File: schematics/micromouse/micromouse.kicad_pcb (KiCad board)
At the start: 2 copper layers, 207.5 x 125.6 mm, 13 parts, among them J1 TOF_FRONT, J2 TOF_LEFT, J3 TOF_RIGHT, J4 Conn_01x06, J5 BatteryConnector, U1 STM32F103CBTx, U2 PMW3360DM-T2QU, U3 BMI160, Y1 Crystal

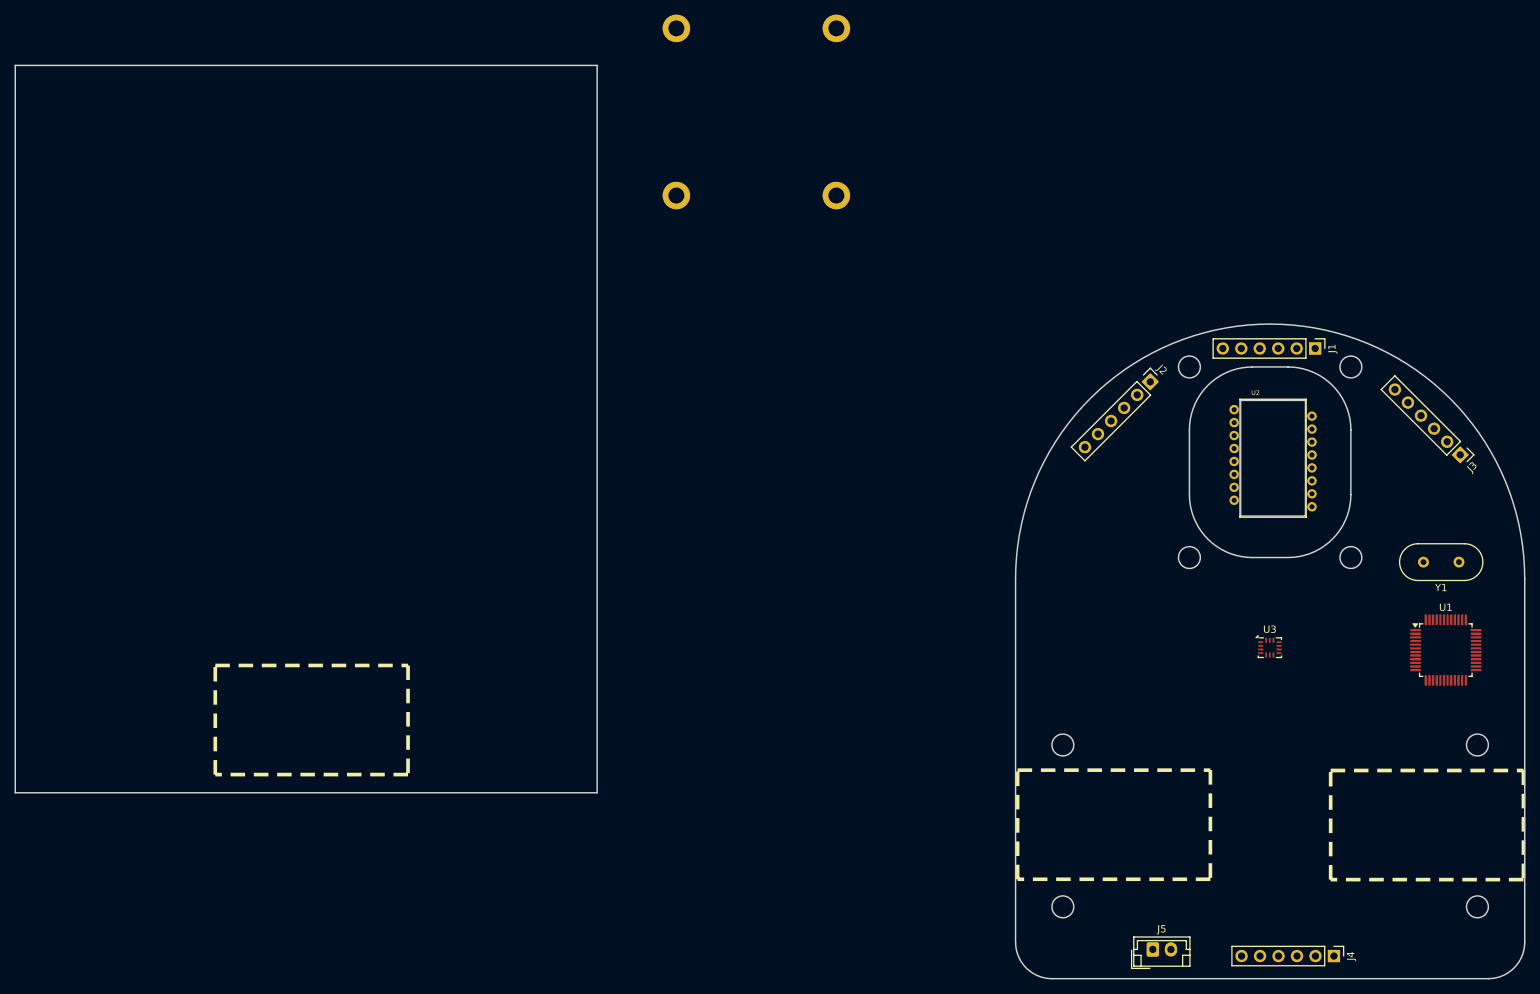
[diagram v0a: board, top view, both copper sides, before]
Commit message: Reorganize again... add things
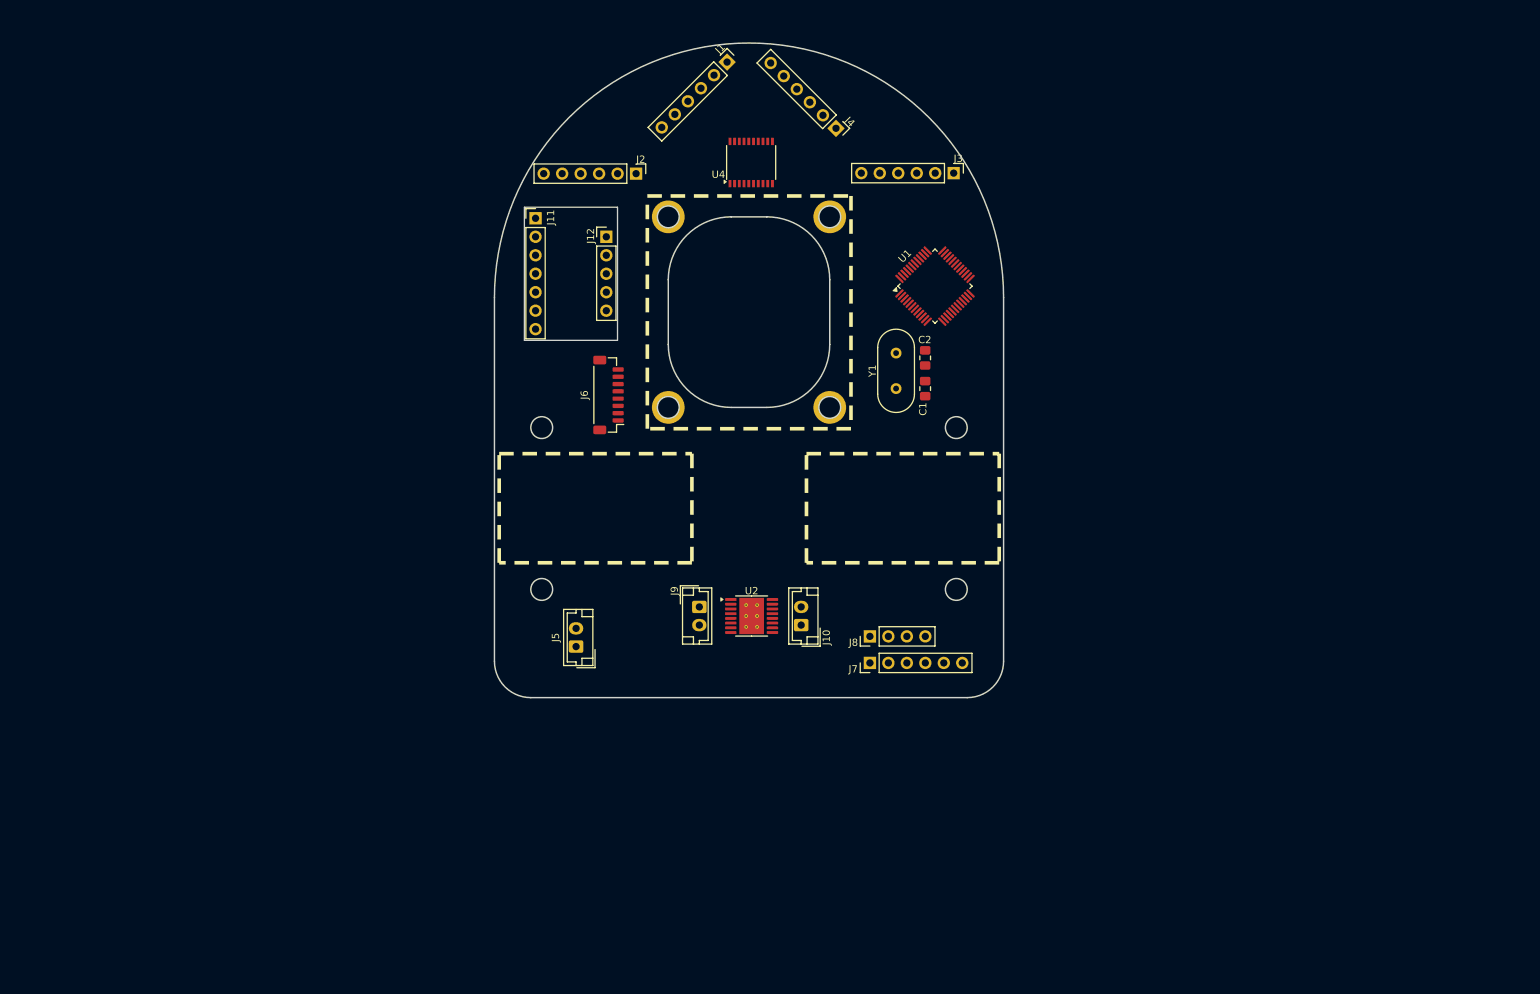
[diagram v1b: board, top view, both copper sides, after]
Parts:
- removed the H1 at (128.4, 42.9)
- removed the H1 at (128.4, 19.9)
- removed the H1 at (150.4, 19.9)
- removed the H1 at (150.4, 42.9)
- removed U3: BMI160, Package_LGA:Bosch_LGA-14_3x2.5mm_P0.5mm
- added C1: C, Capacitor_SMD:C_0805_2012Metric_Pad1.18x1.45mm_HandSolder, F.Cu at (162.6, 69.4)
- added C2: C, Capacitor_SMD:C_0805_2012Metric_Pad1.18x1.45mm_HandSolder, F.Cu at (162.6, 65.2)
- added H1: MountingHole_Pad, MountingHole:MountingHole_2.2mm_M2_ISO14580_Pad, F.Cu at (127.3, 45.8)
- added H2: MountingHole_Pad, MountingHole:MountingHole_2.2mm_M2_ISO14580_Pad, F.Cu at (149.5, 45.8)
- added H3: MountingHole_Pad, MountingHole:MountingHole_2.2mm_M2_ISO14580_Pad, F.Cu at (127.3, 72.0)
- added H4: MountingHole_Pad, MountingHole:MountingHole_2.2mm_M2_ISO14580_Pad, F.Cu at (149.5, 72.0)
- added J10: MotorB_Conn, Connector_JST:JST_EH_B2B-EH-A_1x02_P2.50mm_Vertical, F.Cu at (145.6, 102.0)
- added J11: BMI_ConnB, Connector_PinHeader_2.54mm:PinHeader_1x07_P2.54mm_Vertical, F.Cu at (109.0, 46.0)
- added J12: BMI_ConnA, Connector_PinHeader_2.54mm:PinHeader_1x05_P2.54mm_Vertical, F.Cu at (118.8, 48.6)
- added J4: TOF_RIGHT, Connector_PinHeader_2.54mm:PinHeader_1x06_P2.54mm_Vertical, F.Cu at (150.3, 33.7)
- added J6: PMW3360_Conn, Connector_JST:JST_SH_BM08B-SRSS-TB_1x08-1MP_P1.00mm_Vertical, F.Cu at (119.1, 70.3)
- added J8: Programming_Conn, Connector_PinHeader_2.54mm:PinHeader_1x04_P2.54mm_Vertical, F.Cu at (155.0, 103.5)
- added J9: MotorA_Conn, Connector_JST:JST_EH_B2B-EH-A_1x02_P2.50mm_Vertical, F.Cu at (131.6, 99.5)
- added U4: PCF8574TS, Package_SO:SSOP-20_4.4x6.5mm_P0.65mm, F.Cu at (138.7, 38.4)
- J1: value TOF_FRONT -> TOF_LEFT
- J2: value TOF_LEFT -> TOF_FRONTLEFT
- J3: value TOF_RIGHT -> TOF_FRONTRIGHT
- J7: renamed from J4; value Conn_01x06 -> Bluetooth_Conn
- U2: value PMW3360DM-T2QU -> DRV8833PWP; footprint PMW3360DM:PMW3360 -> Package_SO:HTSSOP-16-1EP_4.4x5mm_P0.65mm_EP3.4x5mm_Mask2.46x2.31mm_ThermalVias
- Y1: value Crystal -> Crystal (8MHz)
- moved J1 89.9 mm to (135.4, 24.5), turned to -45 degrees
- moved J5 89.6 mm to (114.6, 104.9), turned to 90 degrees
- moved U1 86.2 mm to (163.9, 55.4), turned to 45 degrees
- moved Y1 82.6 mm to (158.6, 64.5), turned to -90 degrees
- moved J3 79.7 mm to (166.5, 39.8), turned to -90 degrees
- moved J2 76.3 mm to (122.8, 39.9), turned to -90 degrees
- moved J7 75.5 mm to (155.0, 107.2), turned to 90 degrees
- moved U2 74.9 mm to (138.7, 100.7)
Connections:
- net +3.3V renamed VCC_{3.3}
- net bt_enable renamed /BT_{enable}
- net bt_rx renamed /USART_{RX}
- net bt_state renamed /BT_{state}
- net bt_tx renamed /USART_{TX}
- J1 pad 1: tofF_xshut -> Net-(J1-Pin_1)
- J1 pad 2: tofF_int -> Net-(J1-Pin_2)
- J1 pad 3: tofF_scl -> /I2C2_{scl}
- J1 pad 4: tofF_sda -> /I2C2_{sda}
- J2 pad 1: tofL_xshut -> Net-(J2-Pin_1)
- J2 pad 2: tofL_int -> Net-(J2-Pin_2)
- J2 pad 3: tofL_scl -> /I2C2_{scl}
- J2 pad 4: tofL_sda -> /I2C2_{sda}
- J3 pad 1: tofR_xshut -> Net-(J3-Pin_1)
- J3 pad 2: tofR_int -> Net-(J3-Pin_2)
- J3 pad 3: tofR_scl -> /I2C1_{scl}
- J3 pad 4: tofR_sda -> /I2C1_{sda}
- U1 pad 15: unconnected-(U1-PA5-Pad15) -> /SPI1_{clk}
- U1 pad 16: unconnected-(U1-PA6-Pad16) -> /SPI1_{miso}
- U1 pad 17: unconnected-(U1-PA7-Pad17) -> /SPI1_{mosi}
- U1 pad 21: unconnected-(U1-PB10-Pad21) -> /I2C2_{scl}
- U1 pad 22: unconnected-(U1-PB11-Pad22) -> /I2C2_{sda}
- U1 pad 29: unconnected-(U1-PA8-Pad29) -> /PMW_{cs}
- U1 pad 30: unconnected-(U1-PA9-Pad30) -> /USART1_{TX}
- U1 pad 31: unconnected-(U1-PA10-Pad31) -> /USART1_{RX}
- U1 pad 34: unconnected-(U1-PA13-Pad34) -> /SW_{dio}
- U1 pad 37: unconnected-(U1-PA14-Pad37) -> /SW_{clk}
- U1 pad 42: unconnected-(U1-PB6-Pad42) -> /I2C1_{scl}
- U1 pad 43: unconnected-(U1-PB7-Pad43) -> /I2C1_{sda}
- U1 pad 5: unconnected-(U1-PD0-Pad5) -> Net-(U1-PD0)
- U1 pad 6: unconnected-(U1-PD1-Pad6) -> Net-(U1-PD1)
- U2 pad 1: (no net) -> /MOTOR_{sleep}
- U2 pad 10: unconnected-(U2-SCLK-Pad10) -> /MOTOR_{b2}
- U2 pad 12: unconnected-(U2-MISO-Pad12) -> VCC_{6}
- U2 pad 13: unconnected-(U2-~{CS}-Pad13) -> GND
- U2 pad 14: (no net) -> unconnected-(U2-VINT-Pad14)
- U2 pad 15: unconnected-(U2-LED_P-Pad15) -> /MOTOR_{a2}
- U2 pad 16: (no net) -> /MOTOR_{a1}
- U2 pad 2: (no net) -> Net-(J9-Pin_1)
- U2 pad 3: unconnected-(U2-VDDPIX-Pad3) -> /MOTOR_{aen}
- U2 pad 4: unconnected-(U2-VDD-Pad4) -> Net-(J9-Pin_2)
- U2 pad 5: unconnected-(U2-VDDIO-Pad5) -> Net-(J10-Pin_2)
- U2 pad 6: (no net) -> /MOTOR_{ben}
- U2 pad 7: unconnected-(U2-~{RESET}-Pad7) -> Net-(J10-Pin_1)
- U2 pad 8: unconnected-(U2-GND-Pad8) -> /MOTOR_{fault}
- U2 pad 9: unconnected-(U2-MOTION-Pad9) -> /MOTOR_{b1}
- Y1 pad 1: unconnected-(Y1-Pad1) -> Net-(U1-PD1)
- Y1 pad 2: unconnected-(Y1-Pad2) -> Net-(U1-PD0)
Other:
- board size 207.5 x 125.6 mm -> 70 x 90 mm
- board text removed: "PMW3360 PCB"
